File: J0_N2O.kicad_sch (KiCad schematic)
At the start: 6 parts

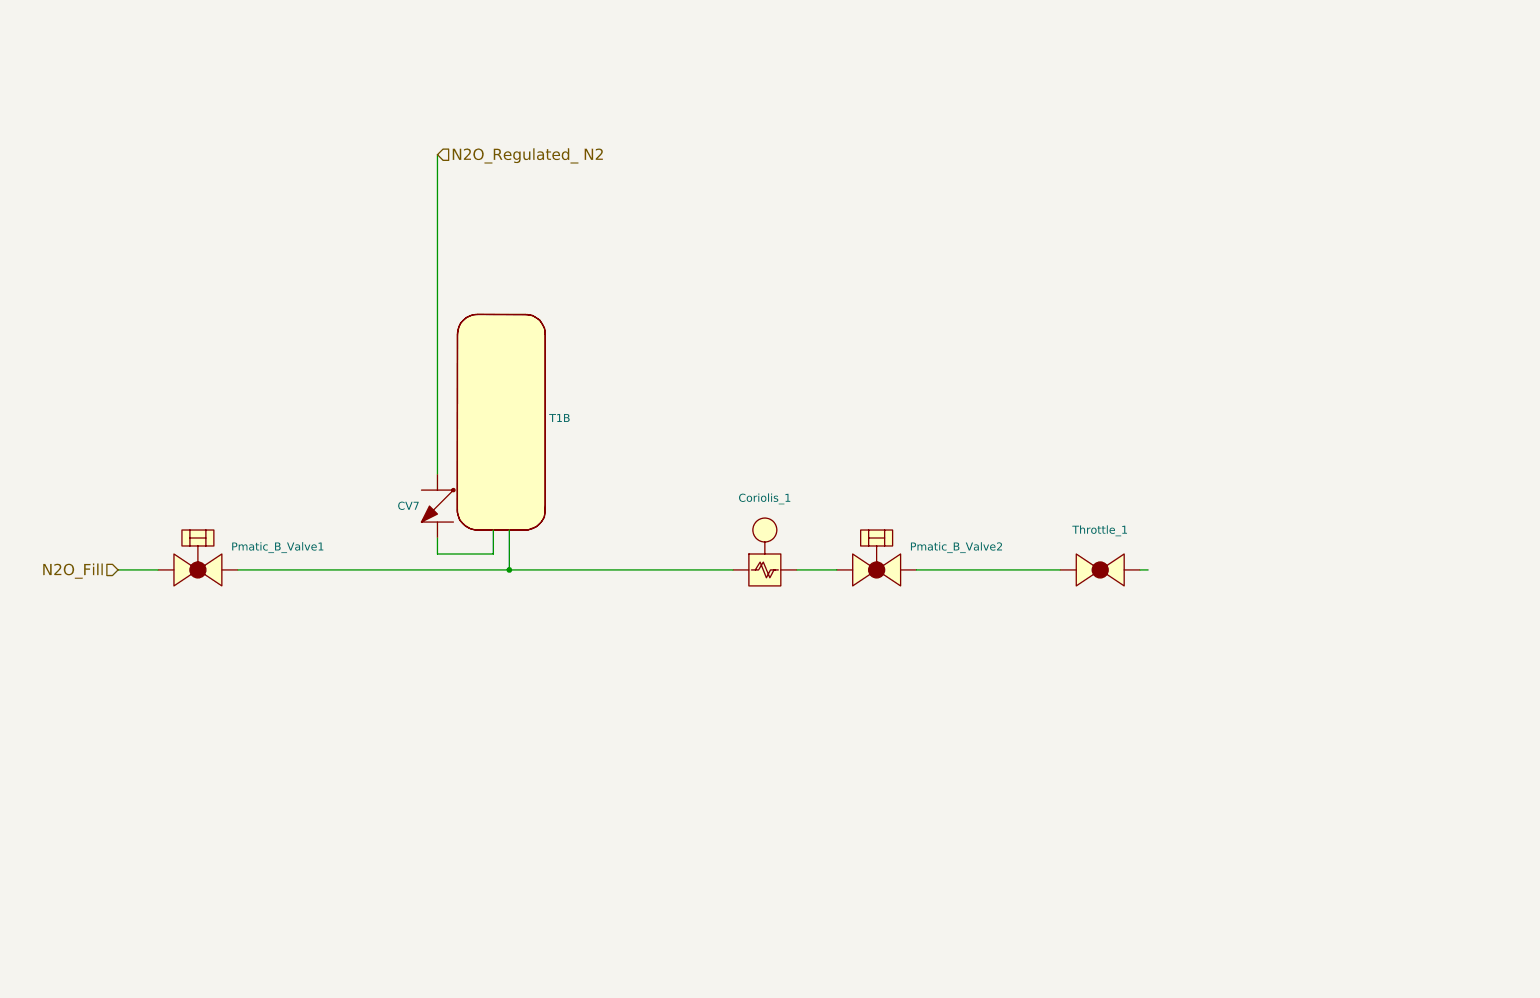
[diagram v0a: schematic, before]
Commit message: andrei it support
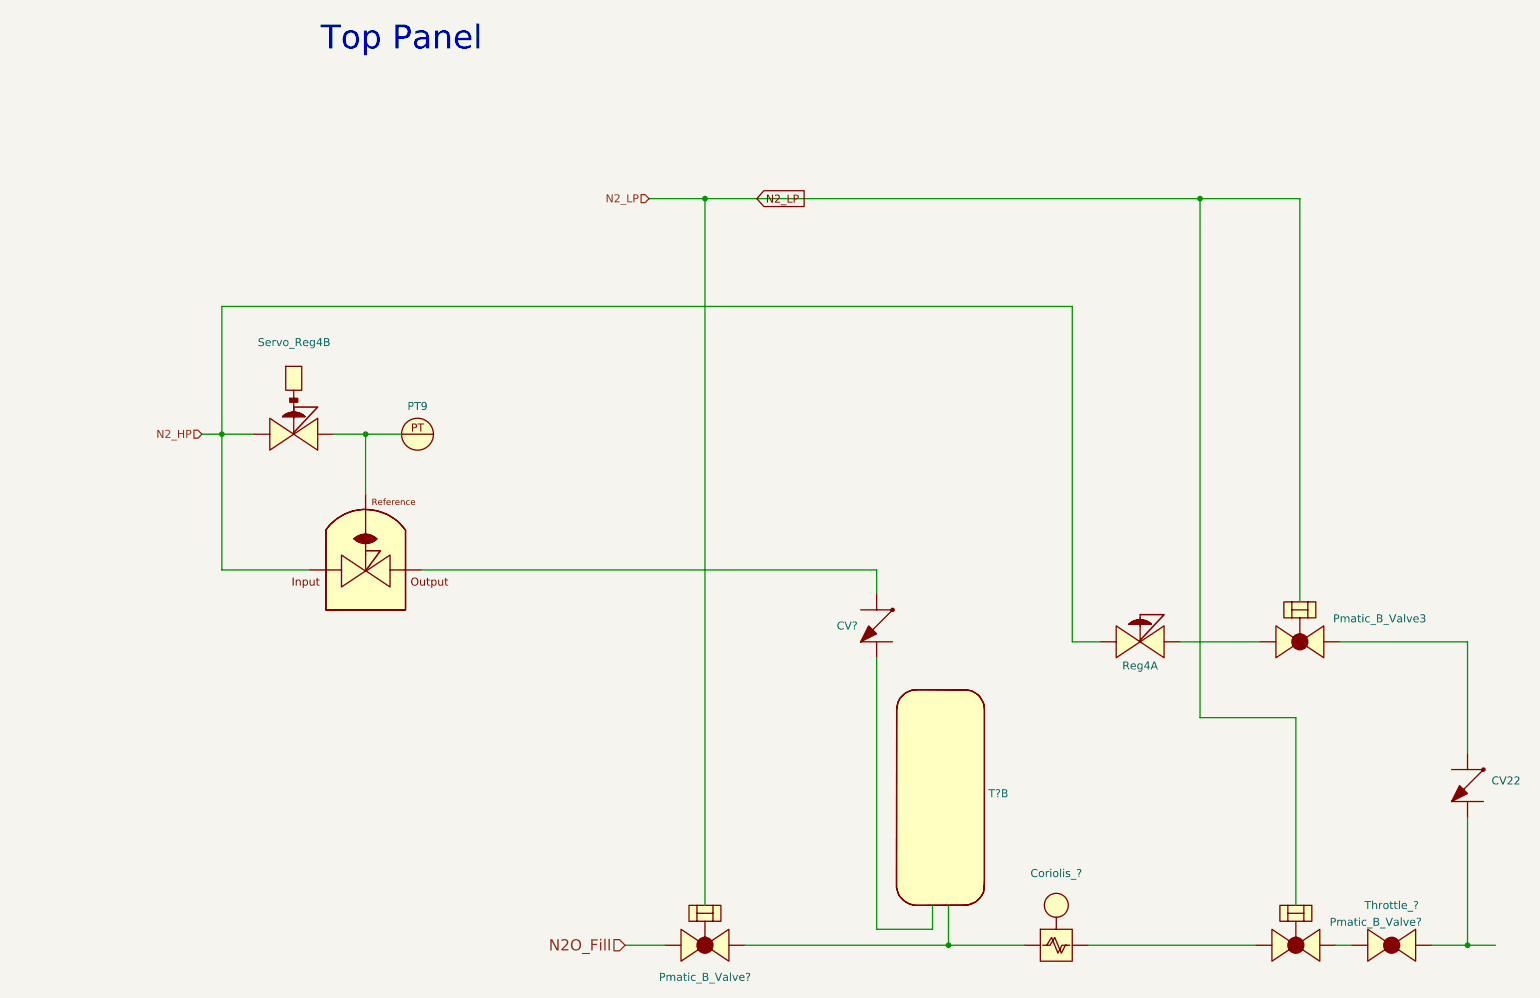
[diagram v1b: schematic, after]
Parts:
- added CV22: ~, symbol PID_symbols:Check_Valve
- added Dome4: ~, symbol PID_symbols:Dome_Reg
- added PT9: ~, symbol PID_symbols:Pressure_Transducer
- added Pmatic_B_Valve3: ~, symbol PID_symbols:Pneumatic_Rotary_Ball_Valve
- added Reg4, Servo_Reg4: ~, symbol PID_symbols:Pressure_Regulator
- renumbered CV7 to CV?, Coriolis_1 to Coriolis_?, Pmatic_B_Valve1 to Pmatic_B_Valve?, Pmatic_B_Valve2 to Pmatic_B_Valve?, T1 to T?, Throttle_1 to Throttle_?
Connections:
- net N2O_Regulated_ N2 is gone; now on an unnamed net: CV?.
- net N2_LP: now reaches Pmatic_B_Valve?.
- net N2_LP: now also Pmatic_B_Valve?., Pmatic_B_Valve3.
- net at Throttle_?.: now also Pmatic_B_Valve?.
- new net: CV?., Dome4.
- new net: Dome4., PT9., Servo_Reg4.
- new net: CV22., Pmatic_B_Valve3.
- new net: CV22., Throttle_?.
- new net: Coriolis_?., Pmatic_B_Valve?., T?.
- new net: Pmatic_B_Valve3., Reg4.
- new net N2_HP: Dome4., Reg4., Servo_Reg4.
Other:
- note added: "Top Panel"
- moved on the sheet: CV?, Coriolis_?, Pmatic_B_Valve?, T?B, Throttle_?
